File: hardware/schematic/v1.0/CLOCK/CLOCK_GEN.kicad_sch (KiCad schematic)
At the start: 147 parts, among them J1 Conn_Coaxial, J10 Conn_Coaxial, J11 Conn_01x06_Socket, J12 Conn_Coaxial, J13 Conn_01x04_Socket, J14 Conn_01x02_Socket, J2 Conn_Coaxial, J3 Conn_Coaxial, J4 Conn_Coaxial, J5 Conn_Coaxial, J6 Conn_Coaxial, J7 Conn_Coaxial, J8 Conn_Coaxial, J9 Conn_Coaxial, U1 LMK5B12204, U2 LMK1C1102, U3 LMK1C1102, U4 TPS78633, U5 TPS78633, U6 OCXO-10M, U7 TPS63020DSJR

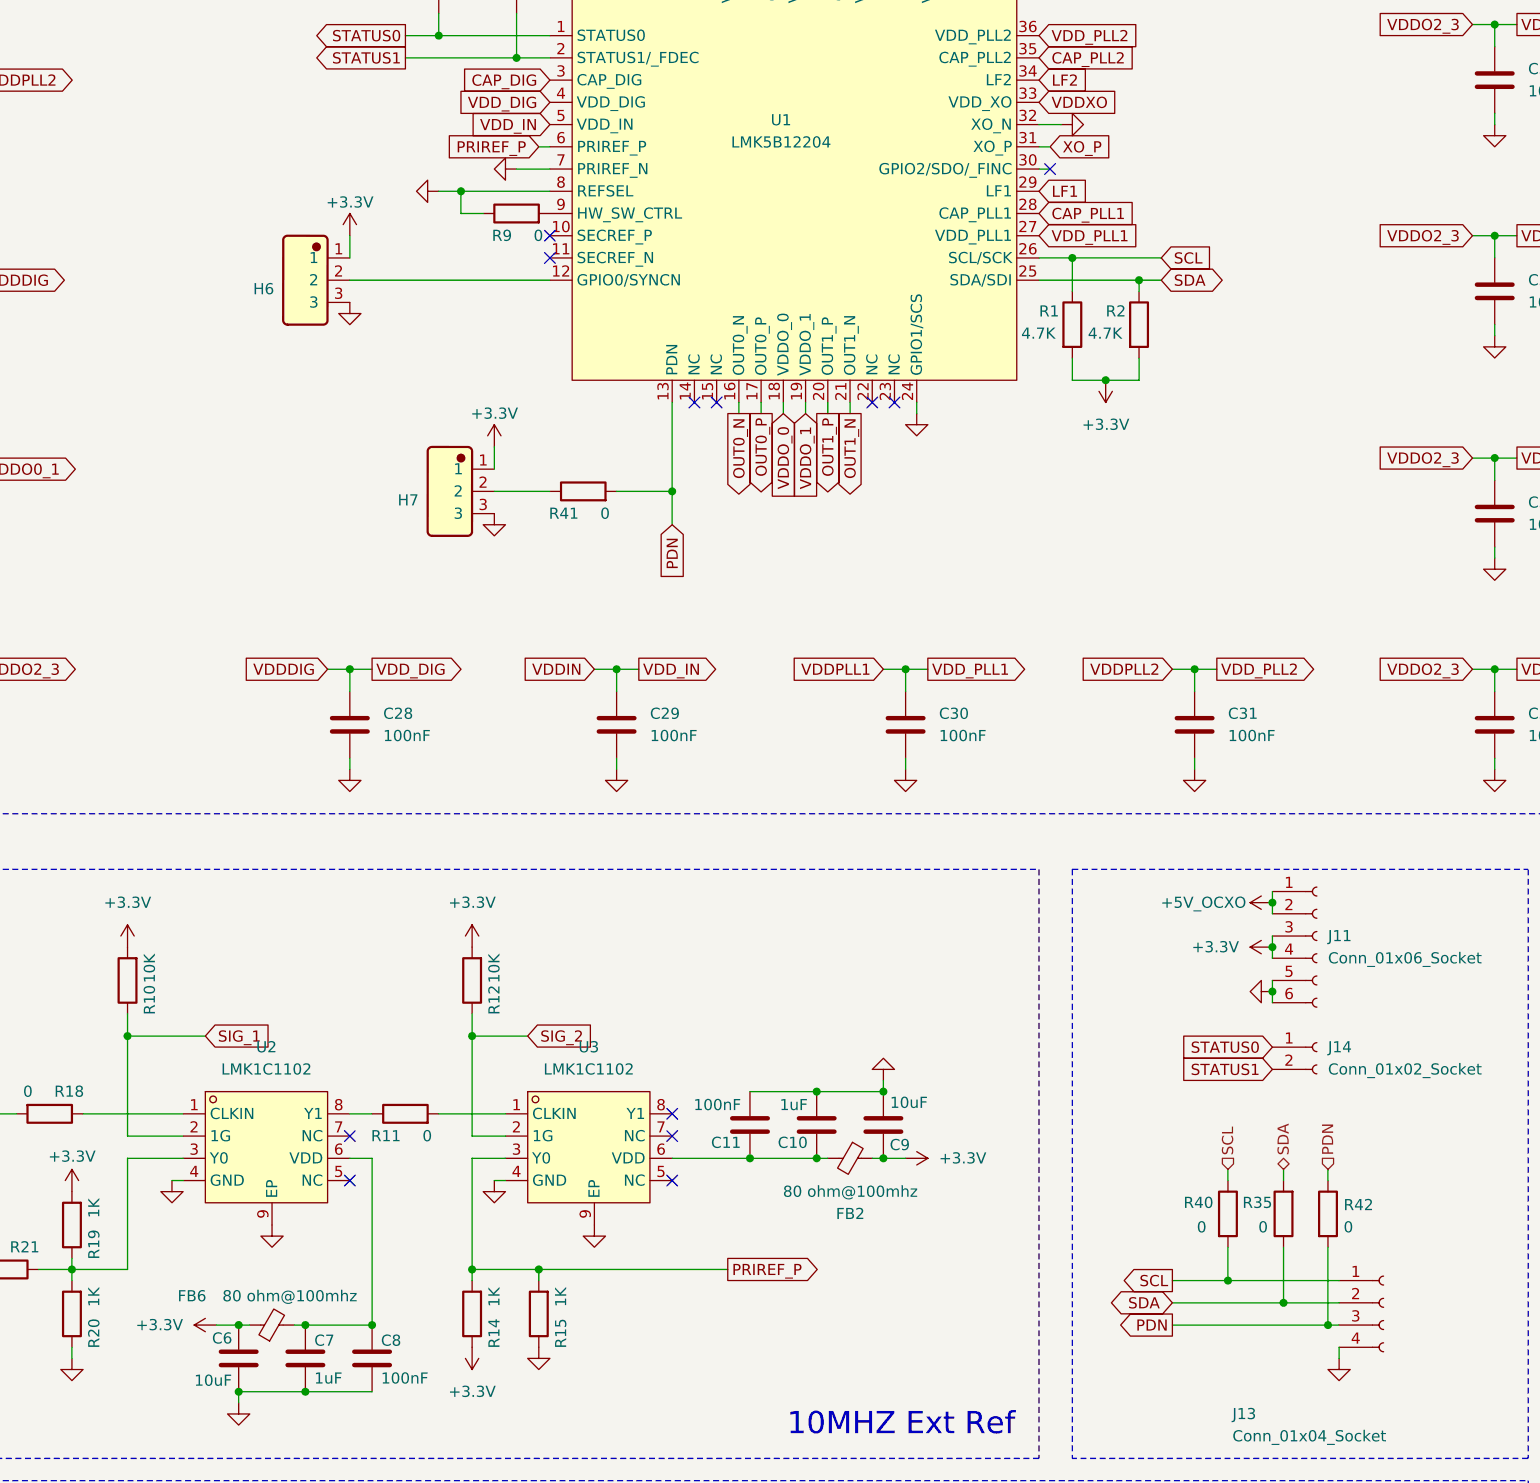
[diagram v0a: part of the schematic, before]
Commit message: sch and pcb update
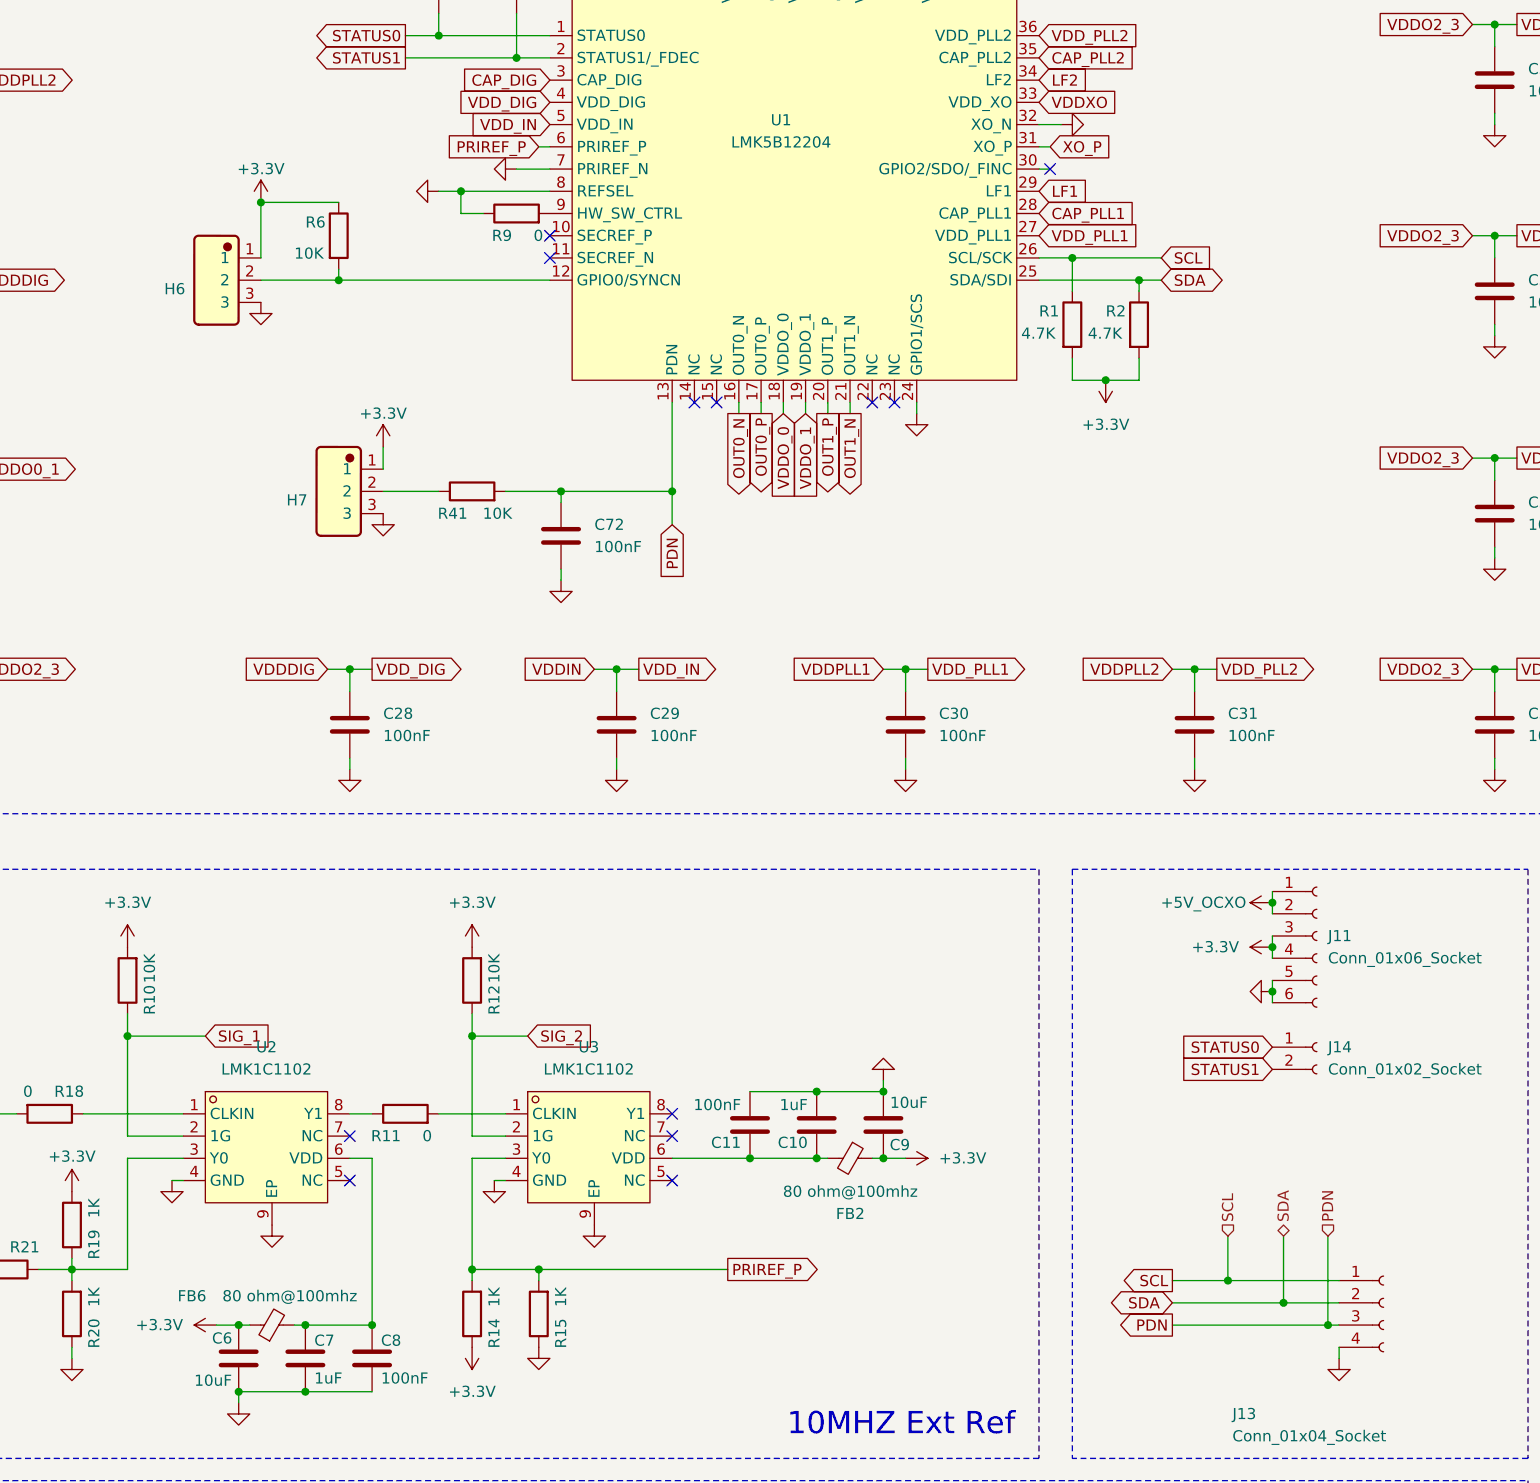
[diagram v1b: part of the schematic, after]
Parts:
- removed R35, R40, R42: 0, Resistor_SMD:R_0402_1005Metric, symbol Device:R
- added C72: 100nF, Capacitor_SMD:C_0402_1005Metric, symbol Device:C
- added R6: 10K, Resistor_SMD:R_0603_1608Metric, symbol Device:R
- R41: value 0 -> 10K
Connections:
- net +3.3V: now also R6.1
- net GND: now also C72.1
- net PDN: now also C72.2
- net at H6.2, U1.12 (GPIO0/SYNCN): now also R6.2
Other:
- moved on the sheet: H6, H7, R41
